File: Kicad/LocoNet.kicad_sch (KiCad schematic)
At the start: 35 parts, among them J1001 Loconet_Power, J1002 Loconet-T, J1003 LN_RX, J1004 LN_TX, J1005 LN_ACT, J1006 Loconet-B, Q1001 BC547, Q1002 BC547, Q1003 BC547, U1001 LM393, U1002 UCC27425

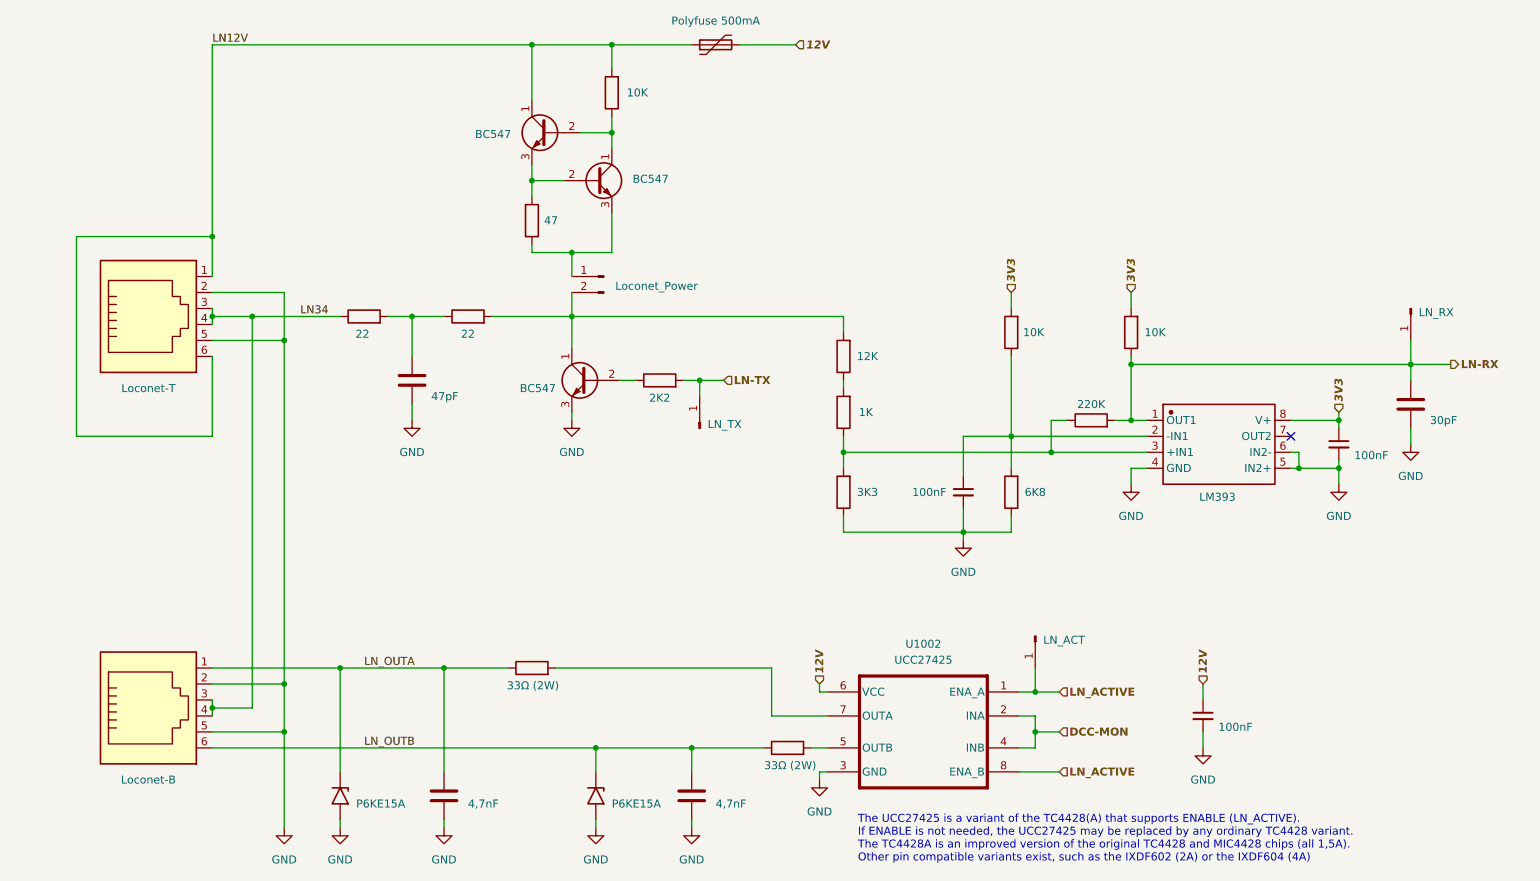
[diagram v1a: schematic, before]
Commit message: Centrale V2.3 (1)
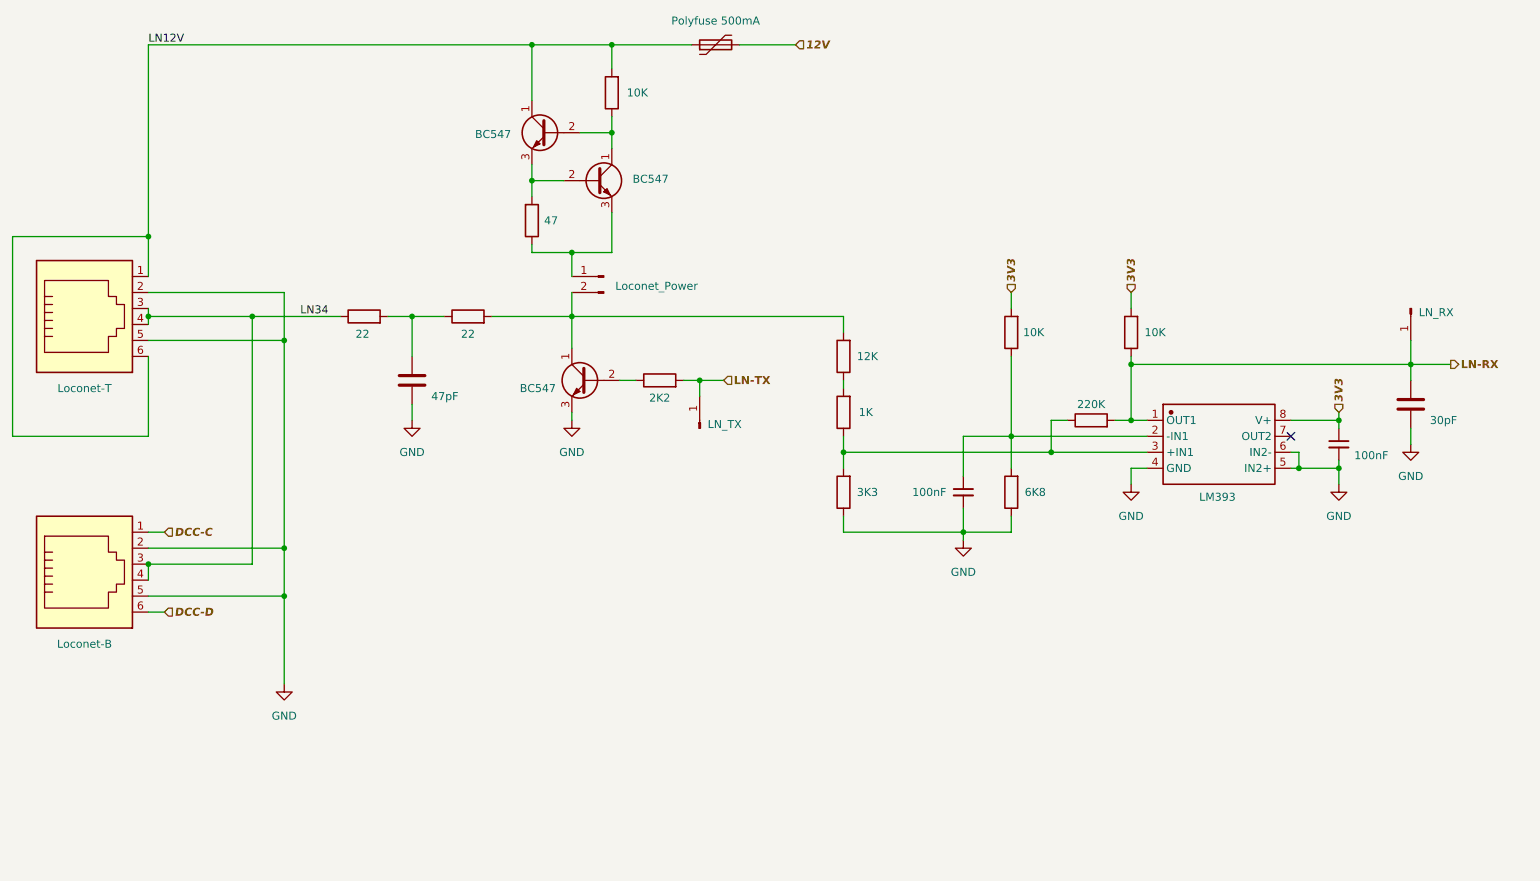
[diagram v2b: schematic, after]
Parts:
- removed C1005: 100nF, Capacitor_THT:C_Disc_D5.0mm_W2.5mm_P2.50mm, symbol Device:C_Small
- removed C1006, C1007: 4,7nF, Capacitor_THT:C_Rect_L10.0mm_W5.0mm_P5.00mm_P7.50mm, symbol Device:C
- removed DTVS1001, DTVS1002: P6KE15A, Diode_THT:D_DO-15_P12.70mm_Horizontal, symbol Diode:5KPxxA
- removed J1005: LN_ACT, Connector_PinHeader_2.54mm:PinHeader_1x01_P2.54mm_Vertical, symbol Connector:Conn_01x01_Pin
- removed R1013, R1014: 33Ω (2W), Resistor_THT:R_Axial_DIN0516_L15.5mm_D5.0mm_P20.32mm_Horizontal, symbol Device:R
- removed U1002: UCC27425, AP_Library:DIL08, symbol AP_Library:UCC27425
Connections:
- net LN_OUTA renamed DCC-C
- net LN_OUTB renamed DCC-D
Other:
- note removed: "The UCC27425 is a variant of the TC4428(A) that supports ENABLE (LN_ACTIVE). If ENABLE is not needed, the UCC27425 may be replaced by any ordinary TC4428 variant. The TC4428A is an improved version of the original TC4428 and MIC4428 chips (all 1,5A). Other pin compatible variants exist, such as the IXDF602 (2A) or the IXDF604 (4A)"
